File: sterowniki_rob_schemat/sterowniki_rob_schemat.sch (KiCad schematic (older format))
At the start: 10 parts, among them Q1 Q_NPN_BCE, U1 STM32L476VGTx, U2 LSM303D

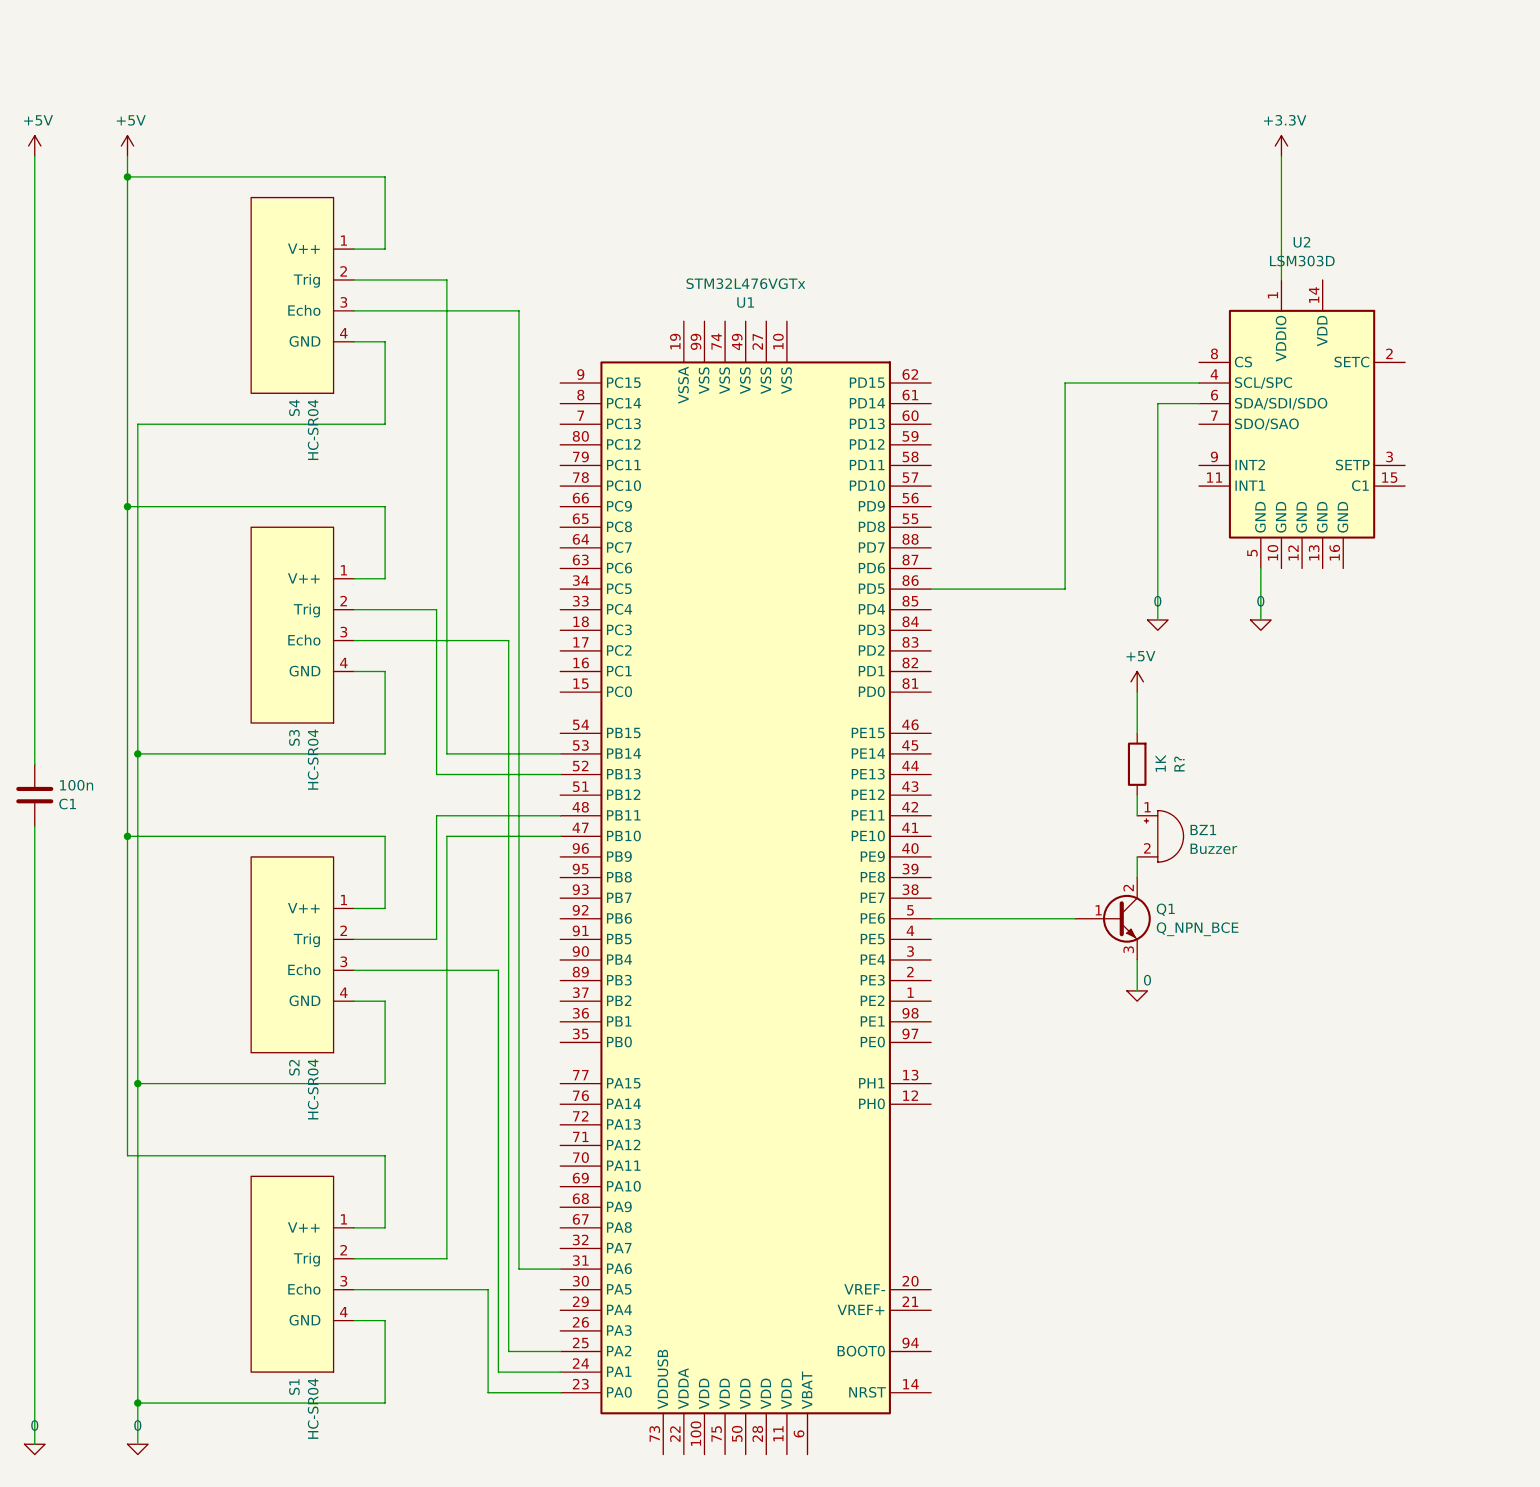
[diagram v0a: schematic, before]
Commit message: schemat v0.2
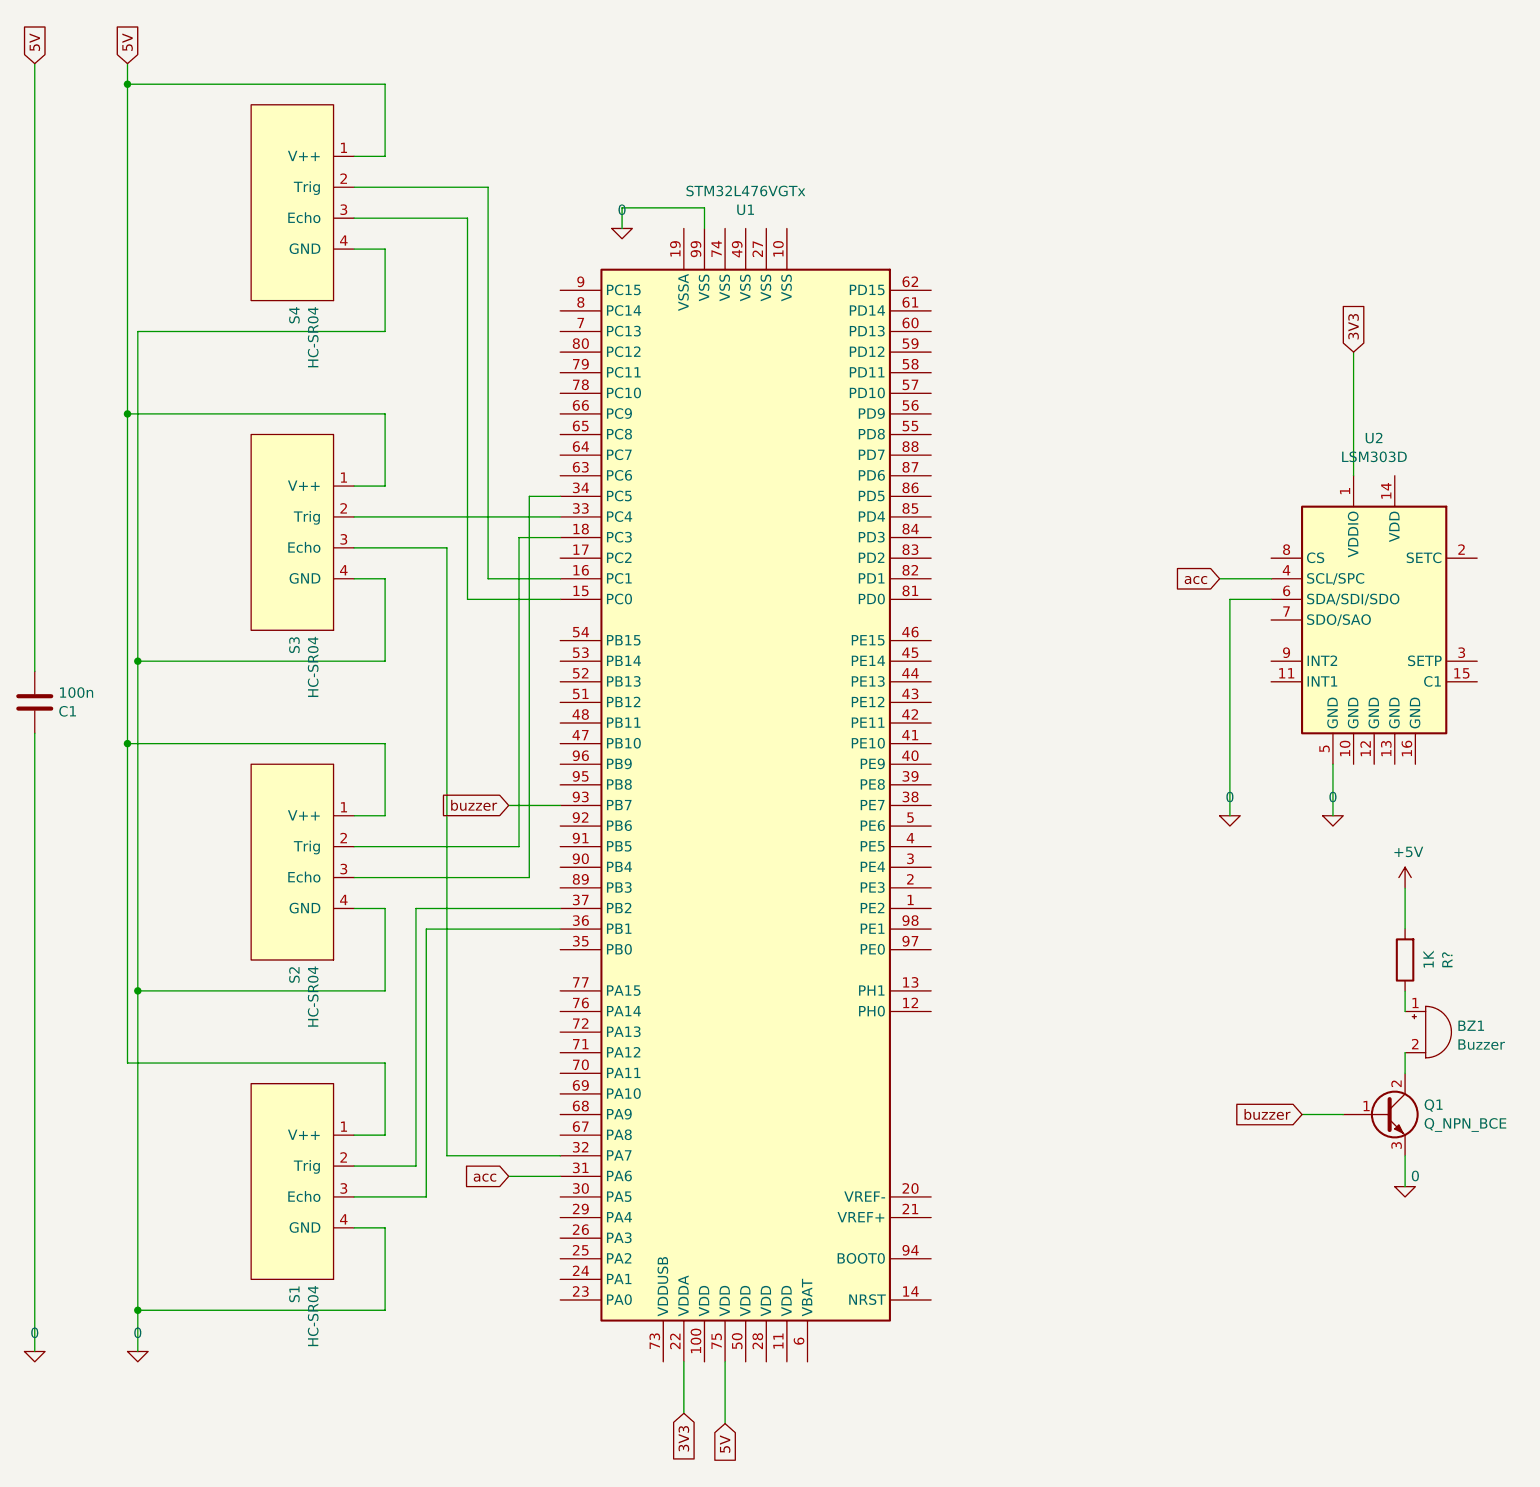
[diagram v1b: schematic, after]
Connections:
- net +3V3 is gone; now on net 3V3: U2.1 (VDDIO)
- net +5V: no longer 100n.1, S1.1 (V++), S2.1 (V++), S3.1 (V++), S4.1 (V++)
- net 0: now also U1.99 (VSS)
- net at S1.2 (Trig): now also U1.37 (PB2); no longer U1.47 (PB10)
- net at S1.3 (Echo): now also U1.36 (PB1); no longer U1.23 (PA0)
- net at U1.86 (PD5): no longer U2.4 (SCL/SPC)
- net at U1.15 (PC0): now also S4.3 (Echo)
- net at U1.16 (PC1): now also S4.2 (Trig)
- net at U1.18 (PC3): now also S2.2 (Trig)
- net 3V3: now reaches U1.22 (VDDA)
- net at U1.24 (PA1): no longer S2.3 (Echo)
- net at U1.25 (PA2): no longer S3.3 (Echo)
- net acc: now reaches U1.31 (PA6)
- net acc: now also U2.4 (SCL/SPC); no longer S4.3 (Echo)
- net at U1.32 (PA7): now also S3.3 (Echo)
- net at U1.33 (PC4): now also S3.2 (Trig)
- net at U1.34 (PC5): now also S2.3 (Echo)
- net at U1.48 (PB11): no longer S2.2 (Trig)
- net at U1.5 (PE6): no longer Q1.1 (B)
- net at U1.52 (PB13): no longer S3.2 (Trig)
- net at U1.53 (PB14): no longer S4.2 (Trig)
- net 5V: now reaches U1.75 (VDD)
- net 5V: now also 100n.1, S1.1 (V++), S2.1 (V++), S3.1 (V++), S4.1 (V++)
- net buzzer: now reaches U1.93 (PB7)
- net buzzer: now also Q1.1 (B)
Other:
- moved on the sheet: 100n, BZ1, Q1, R?, S1, S2, S3, S4, U1, U2

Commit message: schemat polaczen etap II
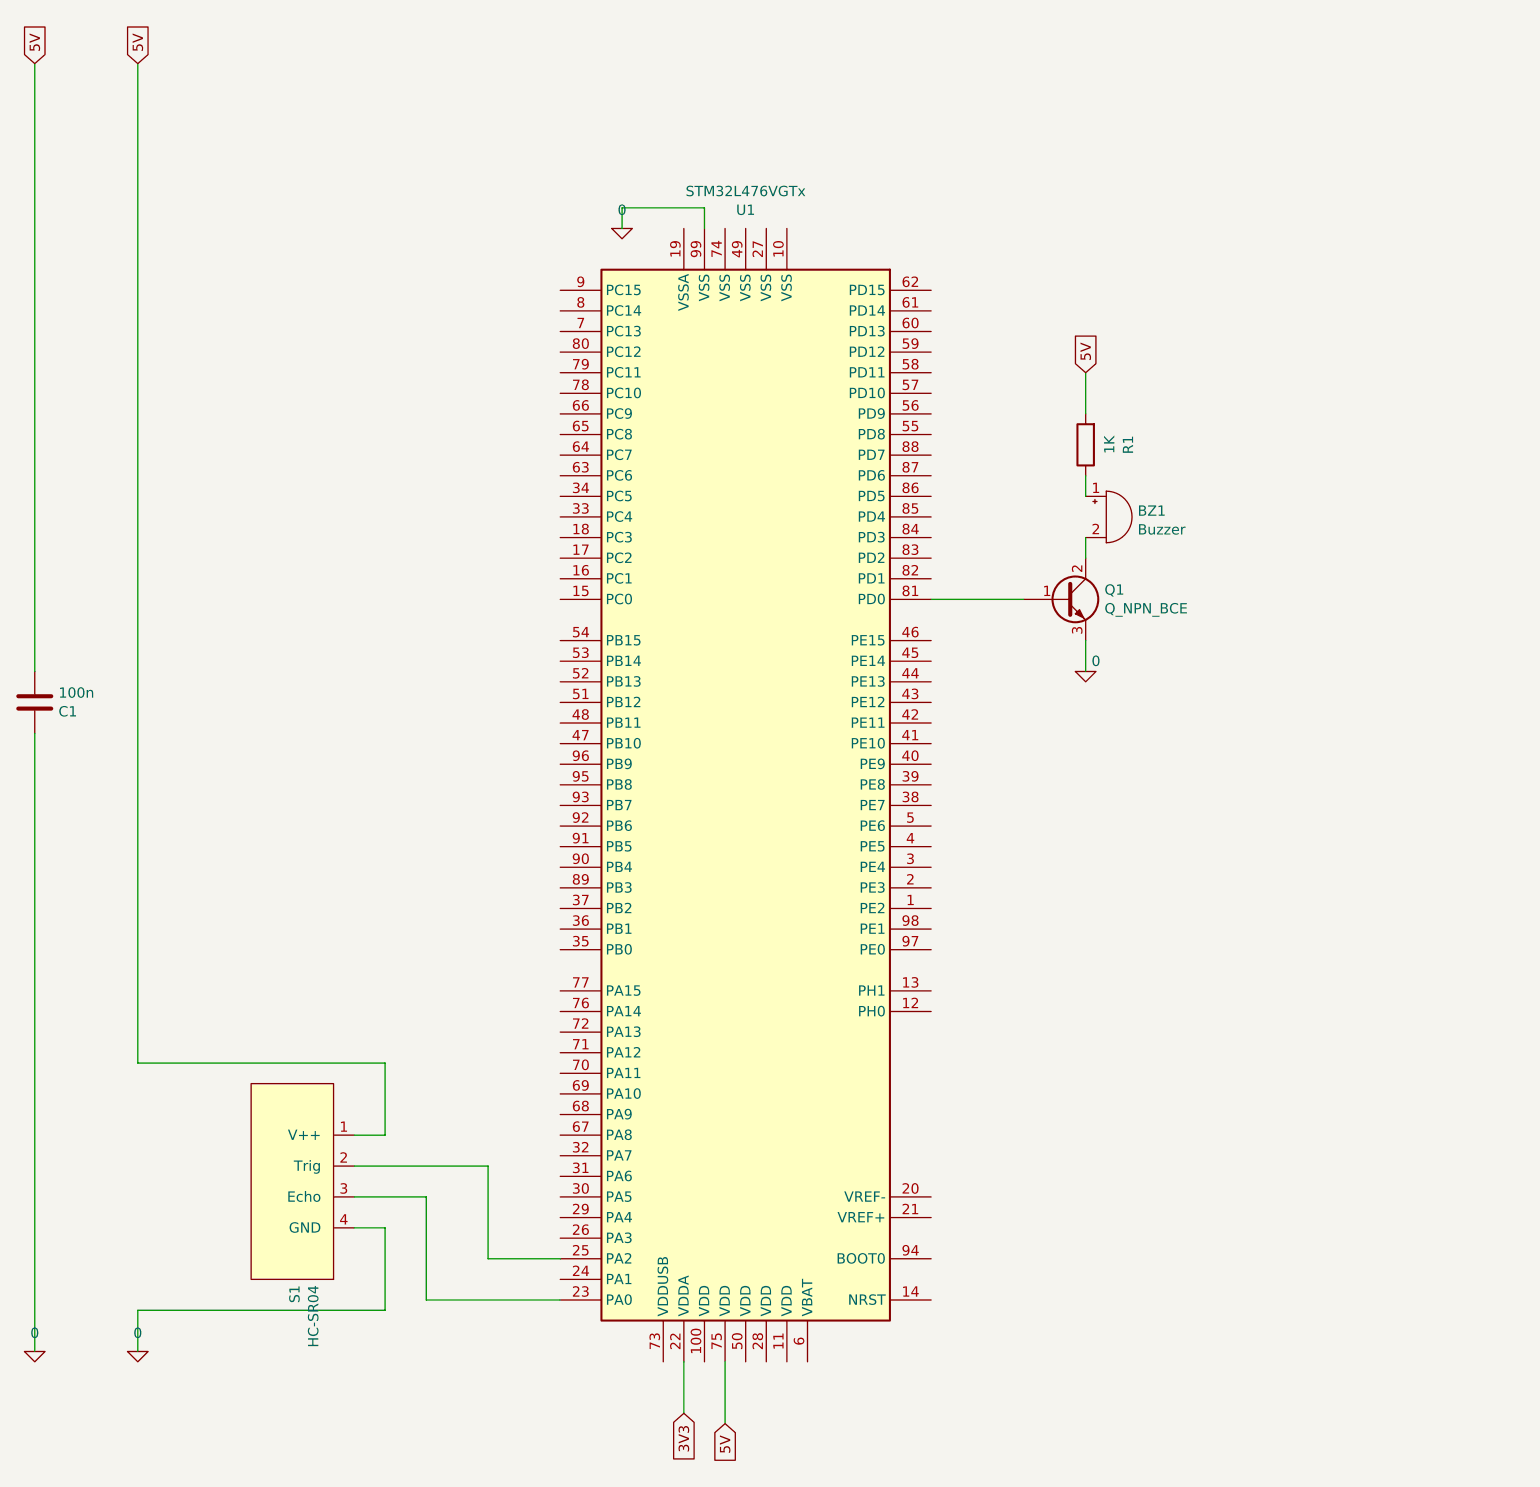
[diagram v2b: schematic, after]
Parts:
- removed S2, S3, S4: HC-SR04, symbol bib:HC-SR04
- removed U2: LSM303D, Package_LGA:LGA-16_3x3mm_P0.5mm, symbol Sensor_Motion:LSM303D
- gave numbers to parts that had none: 1
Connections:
- net +5V is gone; now on net 5V: R1.2
- net at S1.2 (Trig): now also U1.25 (PA2); no longer U1.37 (PB2)
- net at S1.3 (Echo): now also U1.23 (PA0); no longer U1.36 (PB1)
- net at U1.81 (PD0): now also Q1.1 (B)
- net acc: no longer names the net of U1.31 (PA6)
- net buzzer: no longer names the net of U1.93 (PB7)
- net buzzer: no longer Q1.1 (B)
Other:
- moved on the sheet: BZ1, Q1, R1
